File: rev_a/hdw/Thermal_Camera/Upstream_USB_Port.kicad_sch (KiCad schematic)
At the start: 24 parts

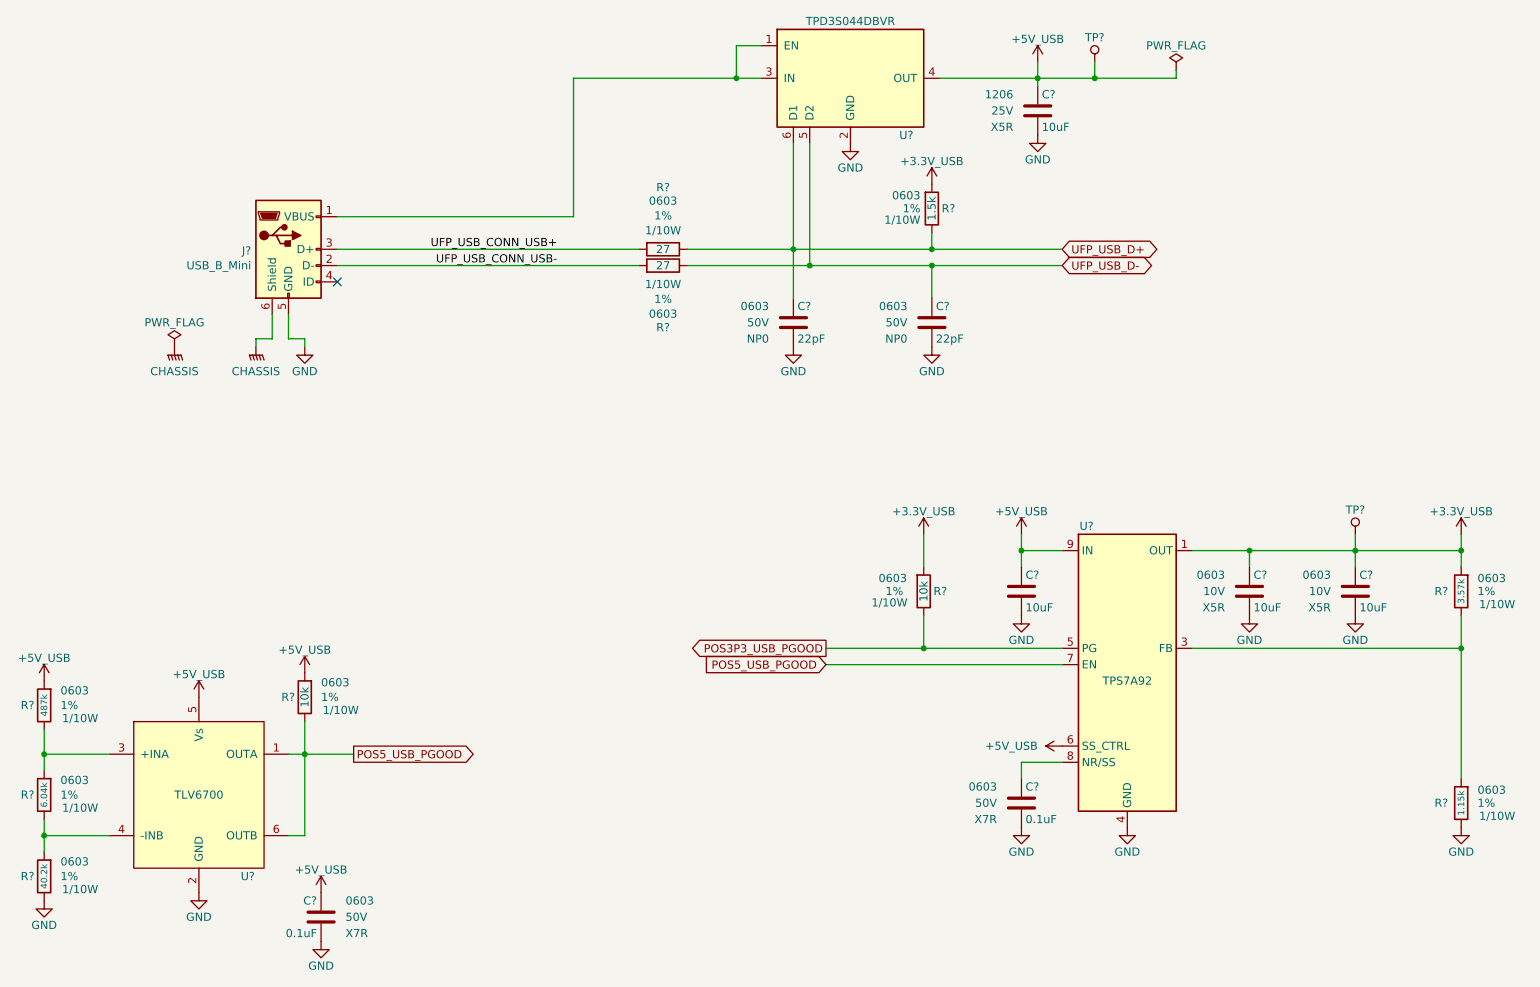
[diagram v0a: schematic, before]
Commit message: lots of random schematic progress
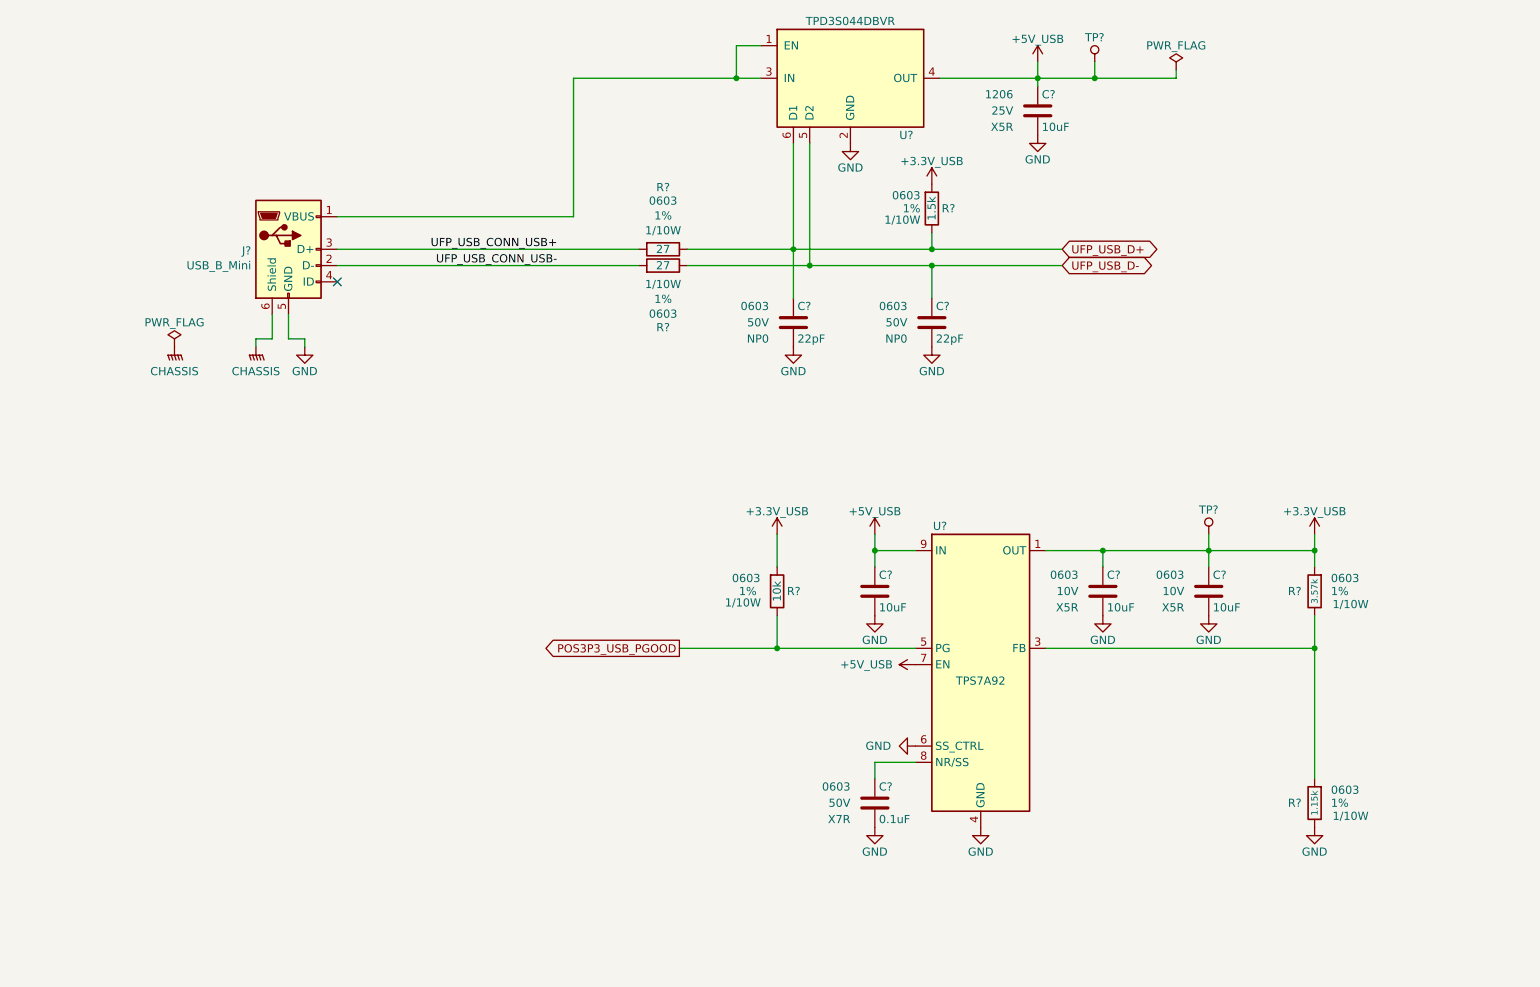
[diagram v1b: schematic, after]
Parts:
- removed C?: 0.1uF, Capacitors_SMD:C_0603, symbol Custom_Library:C_Custom
- removed R?: 487k, Resistors_SMD:R_0603, symbol Custom_Library:R_Custom
- removed R?: 6.04k, Resistors_SMD:R_0603, symbol Custom_Library:R_Custom
- removed R?: 10k, Resistors_SMD:R_0603, symbol Custom_Library:R_Custom
- removed R?: 40.2k, Resistors_SMD:R_0603, symbol Custom_Library:R_Custom
- removed U?: TLV6700, Package_TO_SOT_SMD:SOT-23-6, symbol Custom_Library:TLV6700
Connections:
- net POS5_USB_PGOOD is gone; now on net +5V_USB: U?.7 (EN)
- net +5V_USB: no longer U?.6 (SS_CTRL)
- net GND: now also U?.6 (SS_CTRL)
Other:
- moved on the sheet: C?, R?, TP?, U?
